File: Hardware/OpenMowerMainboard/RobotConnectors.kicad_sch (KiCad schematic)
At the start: 42 parts, among them J1 Conn_02x11_Top_Bottom, J10 Conn_01x05, J11 Conn_01x03_Male, J12 Conn_01x03_Male, J13 Conn_01x03_Male, J14 Conn_01x03_Male, J15 Conn_01x02_Male, J17 Conn_01x02, J18 Conn_01x02, J19 Conn_01x04, J2 Conn_02x04_Top_Bottom, J3 Conn_01x02, J5 Conn_01x04, J6 Conn_01x04, J7 Conn_01x04, J8 Conn_01x04, J9 Conn_01x04

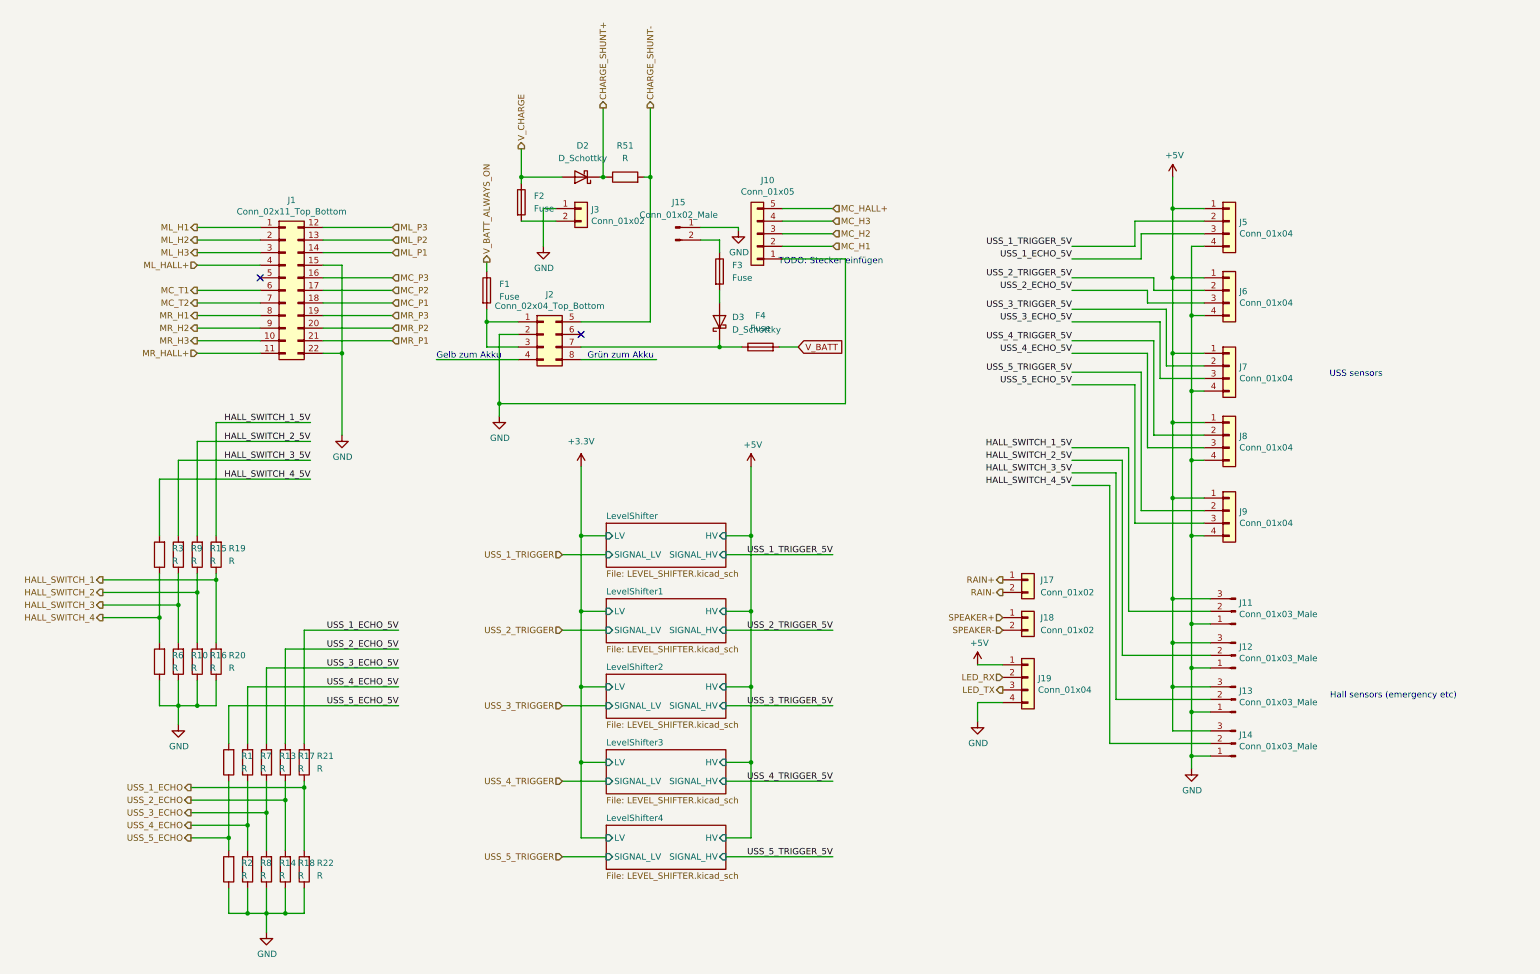
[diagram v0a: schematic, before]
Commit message: added footprints to schematic
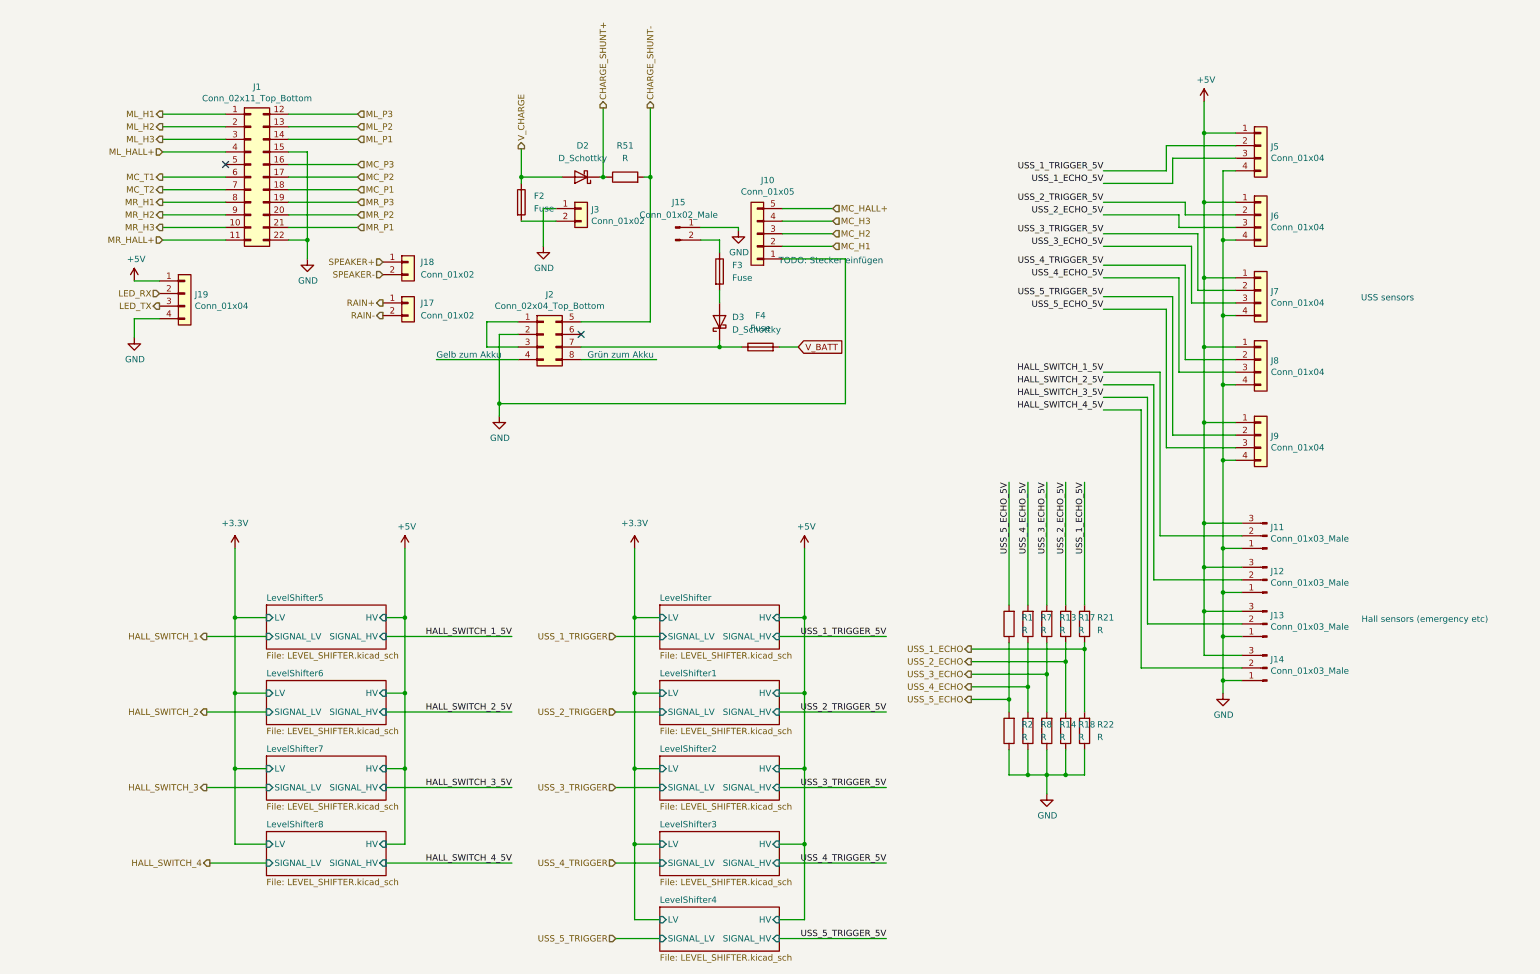
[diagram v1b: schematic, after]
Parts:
- removed F1: Fuse, MyModules:Fuseholder5x20_horiz_open_inline_Type-I, symbol Device:Fuse
- removed R10, R15, R16, R19, R20, R3, R6, R9: R, Resistor_SMD:R_0805_2012Metric, symbol Device:R
- D2, D3: footprint (none) -> Diode_SMD:D_SMA_Handsoldering
- R1, R13, R14, R17, R18, R2, R21, R22, R7, R8: footprint Resistor_SMD:R_0805_2012Metric -> Resistor_SMD:R_0805_2012Metric_Pad1.20x1.40mm_HandSolder
- R51: footprint Resistor_SMD:R_Shunt_Vishay_WSK2512_6332Metric_T2.66mm -> Resistor_SMD:R_2512_6332Metric_Pad1.40x3.35mm_HandSolder
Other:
- added sheet LevelShifter5 (LEVEL_SHIFTER.kicad_sch)
- added sheet LevelShifter6 (LEVEL_SHIFTER.kicad_sch)
- added sheet LevelShifter7 (LEVEL_SHIFTER.kicad_sch)
- added sheet LevelShifter8 (LEVEL_SHIFTER.kicad_sch)
- moved on the sheet: J1, J11, J12, J13, J14, J17, J18, J19, J5, J6, J7, J8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

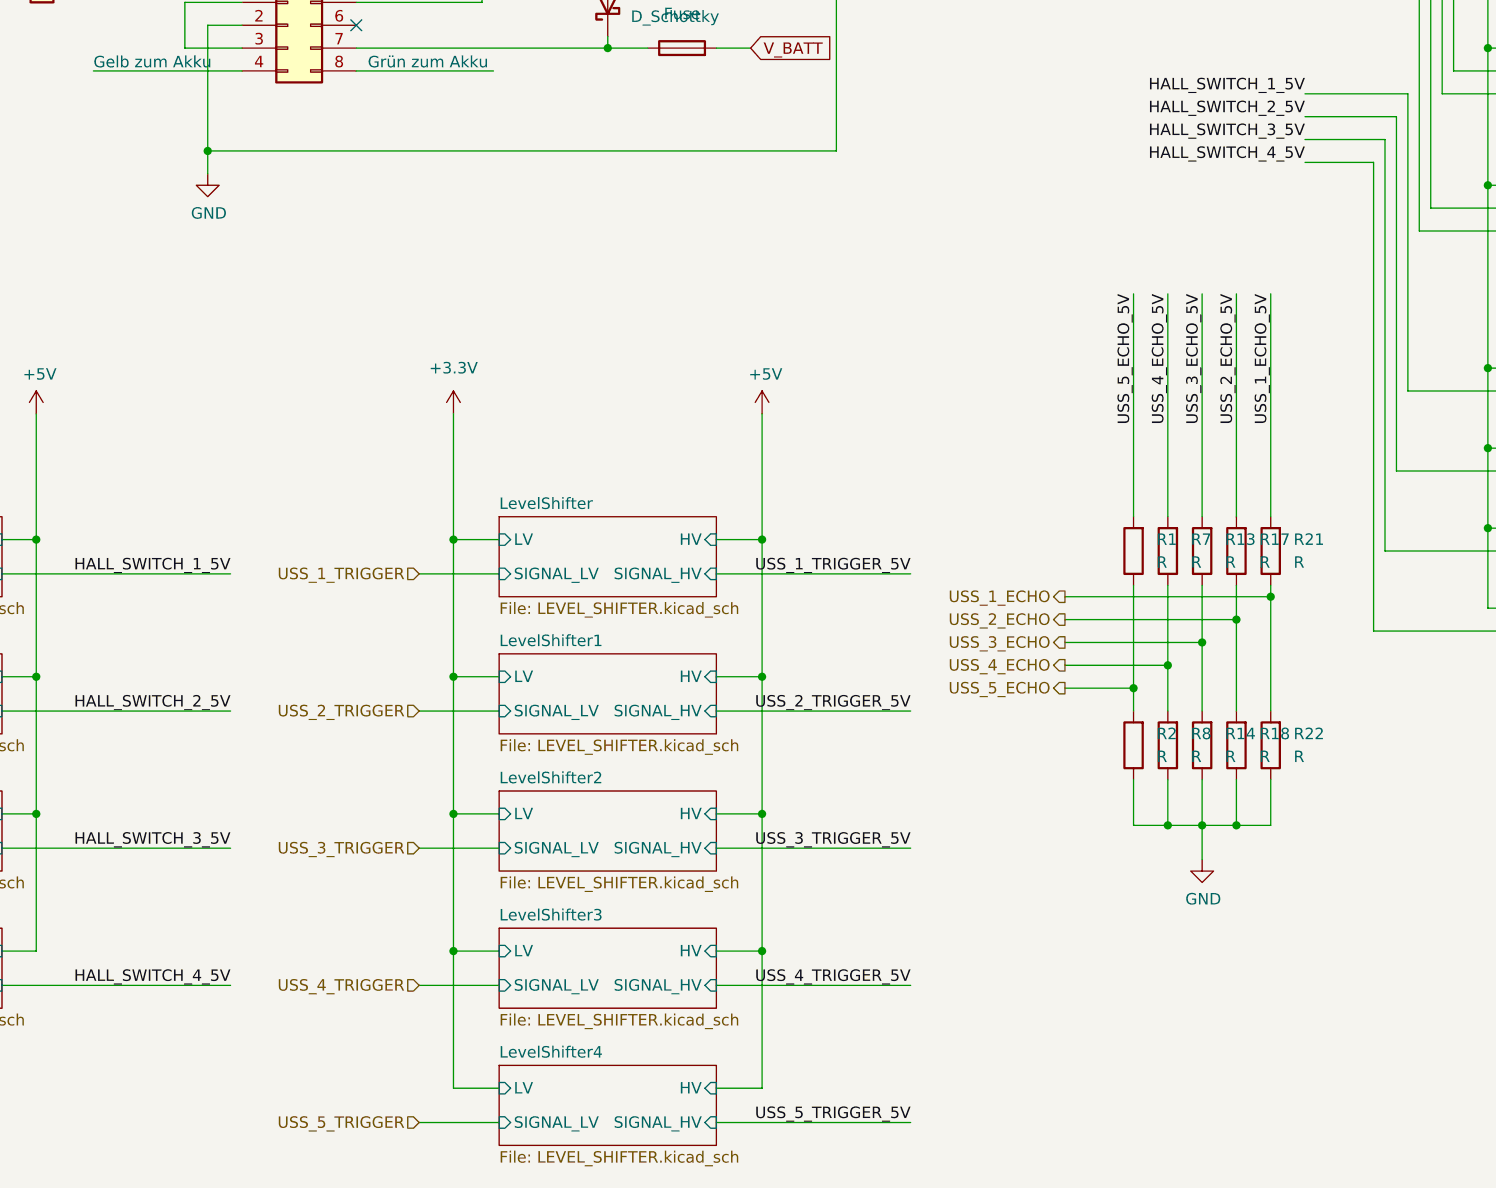
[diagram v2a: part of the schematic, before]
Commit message: wip
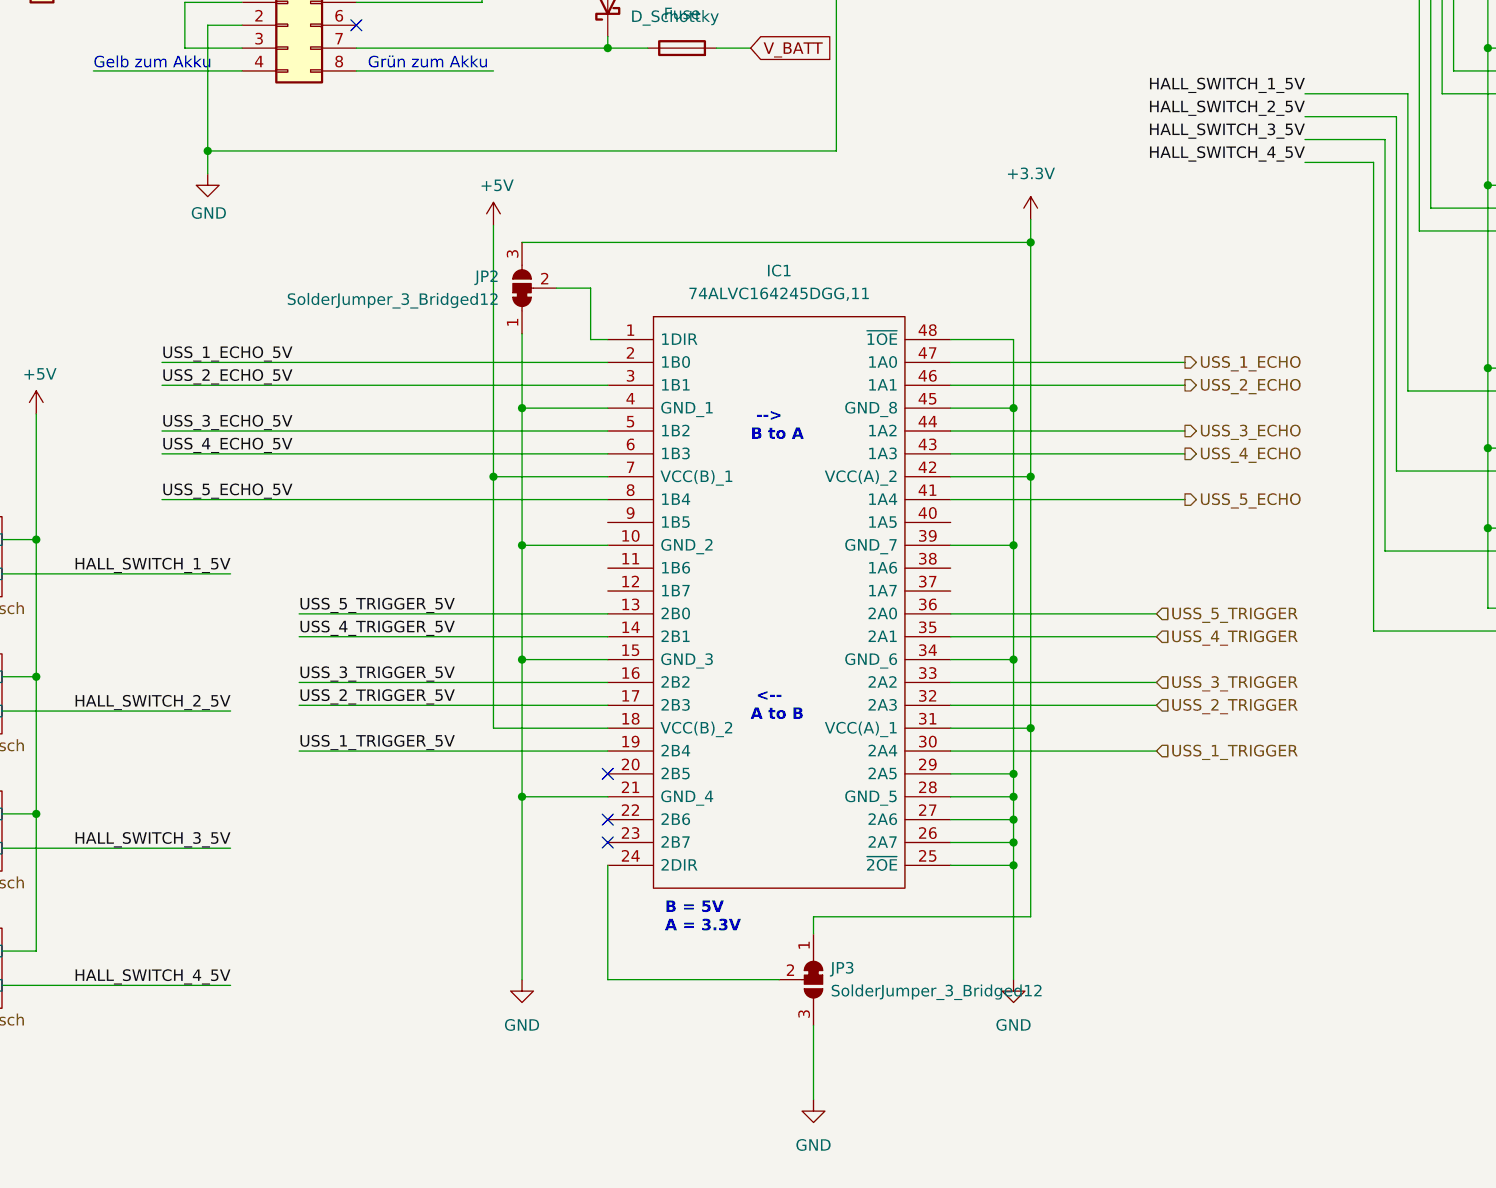
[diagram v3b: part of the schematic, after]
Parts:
- removed R1, R13, R14, R17, R18, R2, R21, R22, R7, R8: R, Resistor_SMD:R_0805_2012Metric_Pad1.20x1.40mm_HandSolder, symbol Device:R
- added IC1: 74ALVC164245DGG,11, SOP50P810X120-48N, symbol 74ALVC164245DGG_11:74ALVC164245DGG,11
- added JP2, JP3: SolderJumper_3_Bridged12, Jumper:SolderJumper-3_P1.3mm_Bridged12_Pad1.0x1.5mm, symbol Jumper:SolderJumper_3_Bridged12
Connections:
- net +3V3: now also IC1.31 (VCC(A)_1), IC1.42 (VCC(A)_2), JP2.3 (B), JP3.1 (A)
- net +5V: now also IC1.18 (VCC(B)_2), IC1.7 (VCC(B)_1)
- net GND: now also IC1.10 (GND_2), IC1.15 (GND_3), IC1.21 (GND_4), IC1.25 (~{2OE}), IC1.26 (2A7), IC1.27 (2A6), IC1.28 (GND_5), IC1.29 (2A5), IC1.34 (GND_6), IC1.39 (GND_7), IC1.4 (GND_1), IC1.45 (GND_8), IC1.48 (~{1OE}), JP2.1 (A), JP3.3 (B)
- net USS_1_ECHO: now also IC1.47 (1A0)
- net USS_1_ECHO_5V: now also IC1.2 (1B0)
- net USS_1_TRIGGER: now also IC1.30 (2A4)
- net USS_1_TRIGGER_5V: now also IC1.19 (2B4)
- net USS_2_ECHO: now also IC1.46 (1A1)
- net USS_2_ECHO_5V: now also IC1.3 (1B1)
- net USS_2_TRIGGER: now also IC1.32 (2A3)
- net USS_2_TRIGGER_5V: now also IC1.17 (2B3)
- net USS_3_ECHO: now also IC1.44 (1A2)
- net USS_3_ECHO_5V: now also IC1.5 (1B2)
- net USS_3_TRIGGER: now also IC1.33 (2A2)
- net USS_3_TRIGGER_5V: now also IC1.16 (2B2)
- net USS_4_ECHO: now also IC1.43 (1A3)
- net USS_4_ECHO_5V: now also IC1.6 (1B3)
- net USS_4_TRIGGER: now also IC1.35 (2A1)
- net USS_4_TRIGGER_5V: now also IC1.14 (2B1)
- net USS_5_ECHO: now also IC1.41 (1A4)
- net USS_5_ECHO_5V: now also IC1.8 (1B4)
- net USS_5_TRIGGER: now also IC1.36 (2A0)
- net USS_5_TRIGGER_5V: now also IC1.13 (2B0)
- new net: IC1.1 (1DIR), JP2.2 (C)
- new net: IC1.24 (2DIR), JP3.2 (C)
- no-connect marks 2 -> 5
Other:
- removed sheet LevelShifter
- removed sheet LevelShifter1
- removed sheet LevelShifter2
- removed sheet LevelShifter3
- removed sheet LevelShifter4
- note added: "--> B to A"
- note added: "<-- A to B"
- note added: "B = 5V A = 3.3V"
